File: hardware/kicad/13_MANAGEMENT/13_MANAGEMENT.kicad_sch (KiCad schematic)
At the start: 6 parts

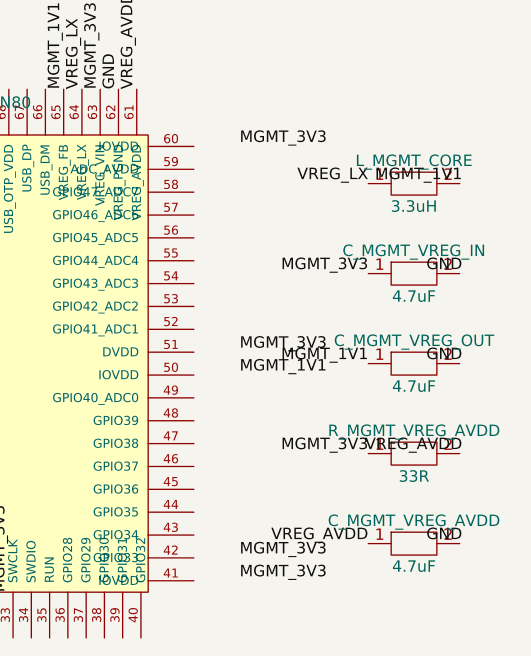
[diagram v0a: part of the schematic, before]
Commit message: M3.7: align Slice A passive labels to native pin endpoints
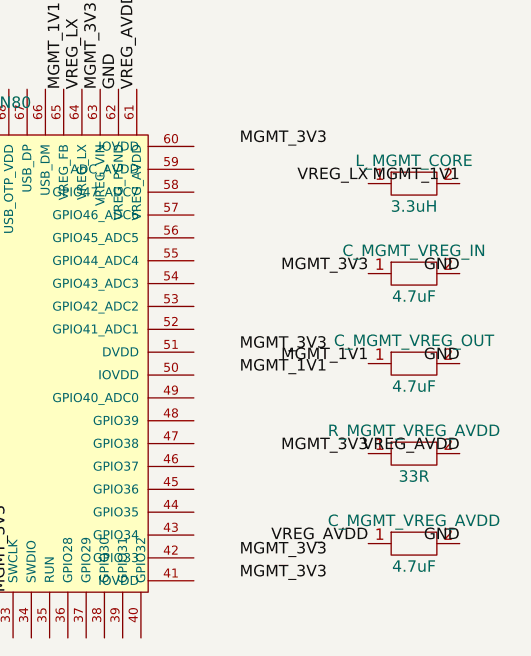
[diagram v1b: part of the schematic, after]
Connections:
- net GND: now also C_MGMT_VREG_AVDD.2, C_MGMT_VREG_IN.2, C_MGMT_VREG_OUT.2
- net MGMT_1V1: now also L_MGMT_CORE.2
- net VREG_AVDD: now also R_MGMT_VREG_AVDD.2
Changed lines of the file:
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@@
   )
   (label "VREG_LX" (at 144.78 80 0) (effects (font (size 1.27 1.27)) (justify right bottom)))
-  (label "MGMT_1V1" (at 155.22 80 180) (effects (font (size 1.27 1.27)) (justify right bottom)))
+  (label "MGMT_1V1" (at 154.94 80 180) (effects (font (size 1.27 1.27)) (justify right bottom)))
   (symbol (lib_id "RetroSBC-management:C_LOCAL") (at 149.86 90 0) (unit 1)
     (exclude_from_sim no) (in_bom yes) (on_board yes)
@@
   )
   (label "MGMT_3V3" (at 144.78 90 0) (effects (font (size 1.27 1.27)) (justify right bottom)))
-  (label "GND" (at 155.22 90 180) (effects (font (size 1.27 1.27)) (justify right bottom)))
+  (label "GND" (at 154.94 90 180) (effects (font (size 1.27 1.27)) (justify right bottom)))
   (symbol (lib_id "RetroSBC-management:C_LOCAL") (at 149.86 100 0) (unit 1)
     (exclude_from_sim no) (in_bom yes) (on_board yes)
@@
   )
   (label "MGMT_1V1" (at 144.78 100 0) (effects (font (size 1.27 1.27)) (justify right bottom)))
-  (label "GND" (at 155.22 100 180) (effects (font (size 1.27 1.27)) (justify right bottom)))
+  (label "GND" (at 154.94 100 180) (effects (font (size 1.27 1.27)) (justify right bottom)))
   (symbol (lib_id "RetroSBC-management:R_LOCAL") (at 149.86 110 0) (unit 1)
     (exclude_from_sim no) (in_bom yes) (on_board yes)
@@
   )
   (label "MGMT_3V3" (at 144.78 110 0) (effects (font (size 1.27 1.27)) (justify right bottom)))
-  (label "VREG_AVDD" (at 155.22 110 180) (effects (font (size 1.27 1.27)) (justify right bottom)))
+  (label "VREG_AVDD" (at 154.94 110 180) (effects (font (size 1.27 1.27)) (justify right bottom)))
   (symbol (lib_id "RetroSBC-management:C_LOCAL") (at 149.86 120 0) (unit 1)
     (exclude_from_sim no) (in_bom yes) (on_board yes)
@@
   )
   (label "VREG_AVDD" (at 144.78 120 0) (effects (font (size 1.27 1.27)) (justify right bottom)))
-  (label "GND" (at 155.22 120 180) (effects (font (size 1.27 1.27)) (justify right bottom)))
+  (label "GND" (at 154.94 120 180) (effects (font (size 1.27 1.27)) (justify right bottom)))
   (label "MGMT_3V3" (at 69.52000000000001 113.97 0)
     (effects (font (size 1.27 1.27)) (justify left bottom))
